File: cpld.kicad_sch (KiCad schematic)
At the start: 2 parts, among them J2 Conn_01x06_Pin, U6 ATF1508AS-10AU100

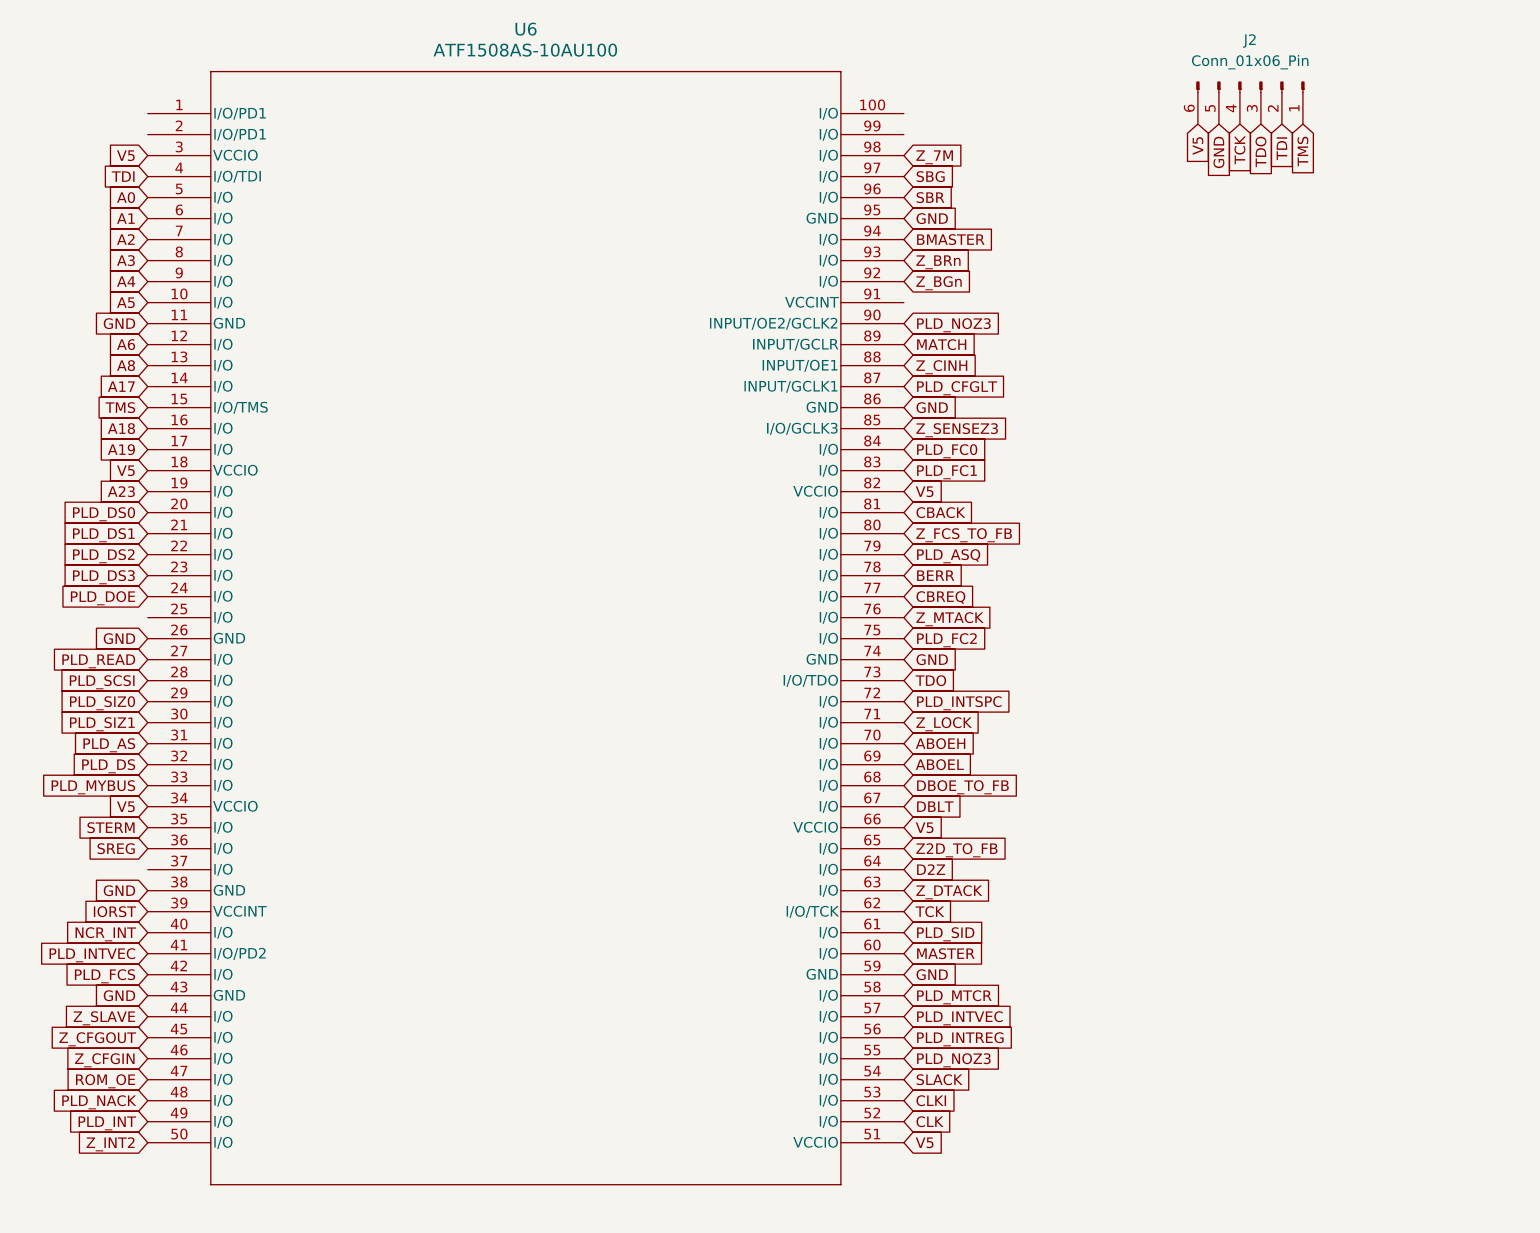
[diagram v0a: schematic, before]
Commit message: More work. Getting there.
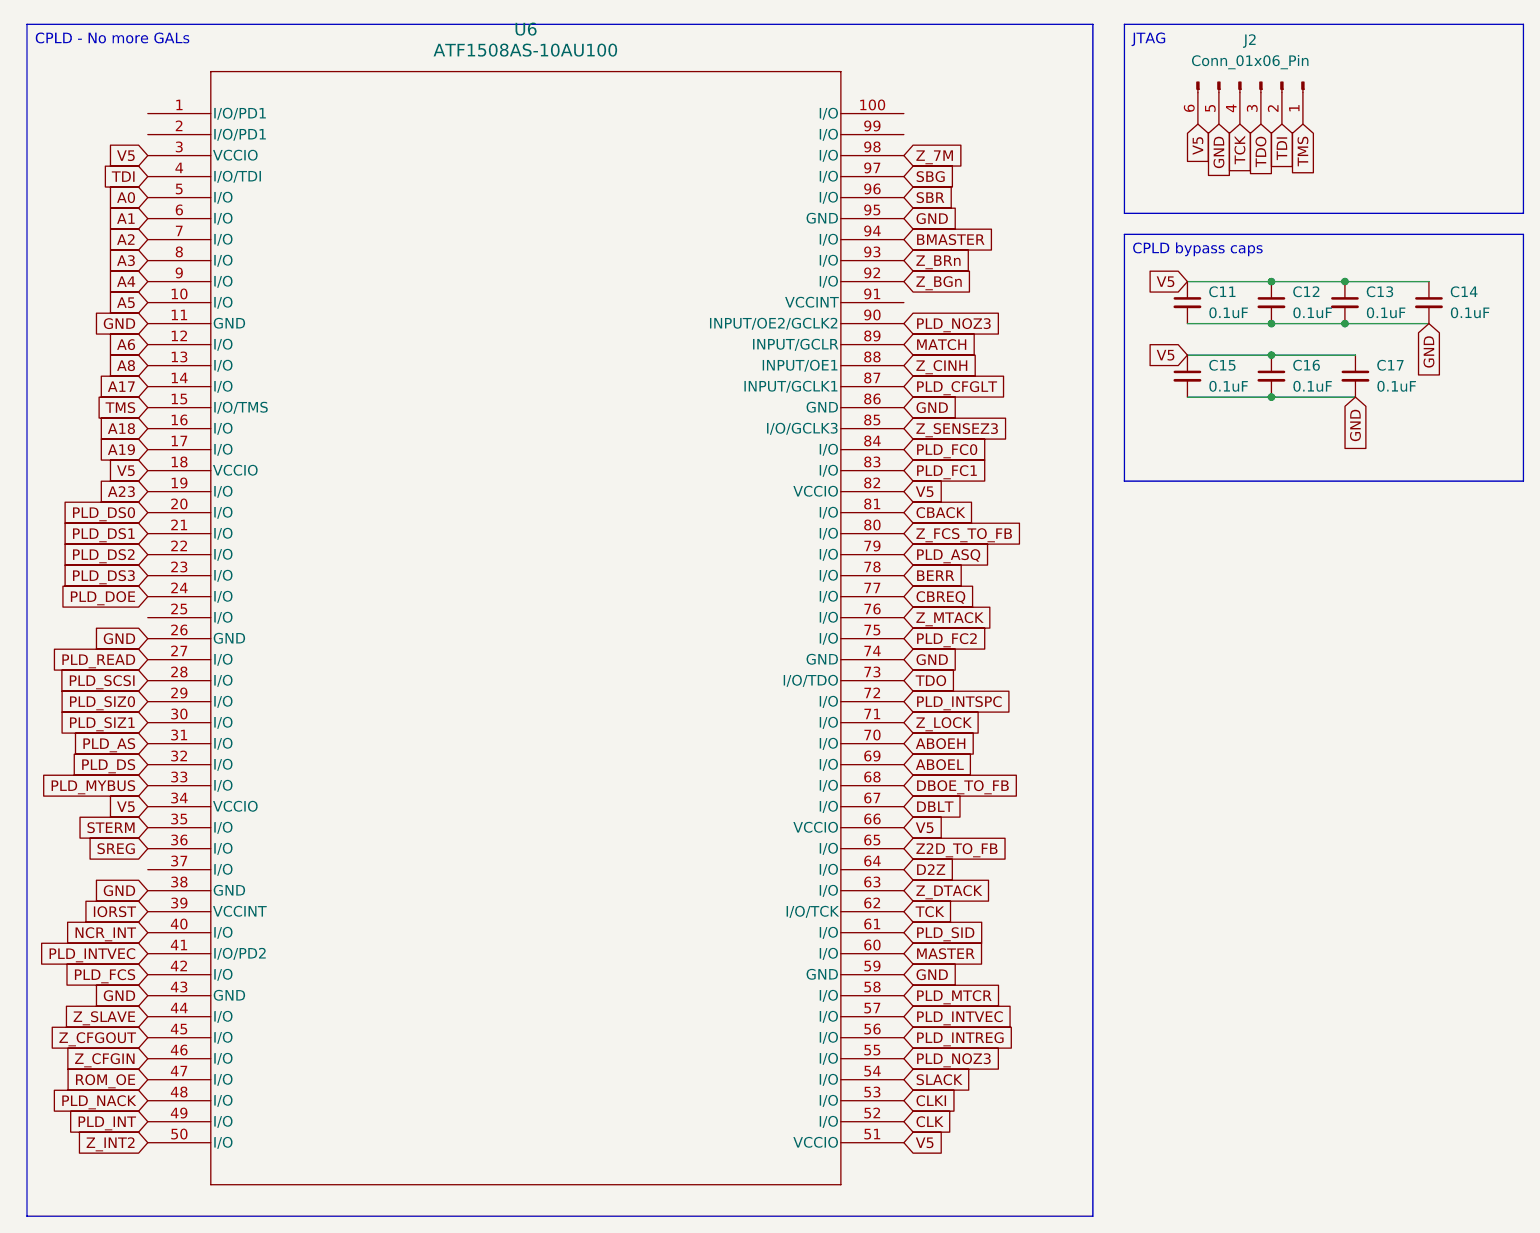
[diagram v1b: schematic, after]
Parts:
- added C11, C12, C13, C14, C15, C16, C17: 0.1uF, symbol Device:C_Small
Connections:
- net GND: now also C11.2, C12.2, C13.2, C14.2, C15.2, C16.2, C17.2
- net V5: now also C11.1, C12.1, C13.1, C14.1, C15.1, C16.1, C17.1
